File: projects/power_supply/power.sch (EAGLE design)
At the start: 82 parts, among them SW1 SRIDE_SWITCH, SW2 SRIDE_SWITCH, SW3 SRIDE_SWITCH, SW4 SRIDE_SWITCH, SW5 SRIDE_SWITCH, SW6 SRIDE_SWITCH, SW7 SRIDE_SWITCH, SW8 SRIDE_SWITCH

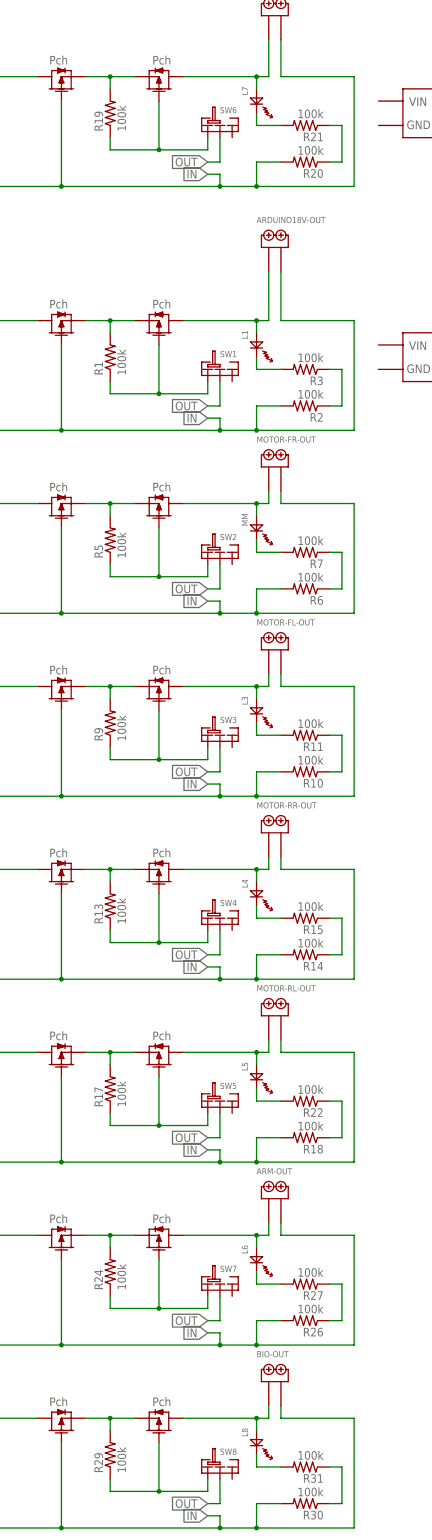
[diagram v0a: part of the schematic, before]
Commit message: power
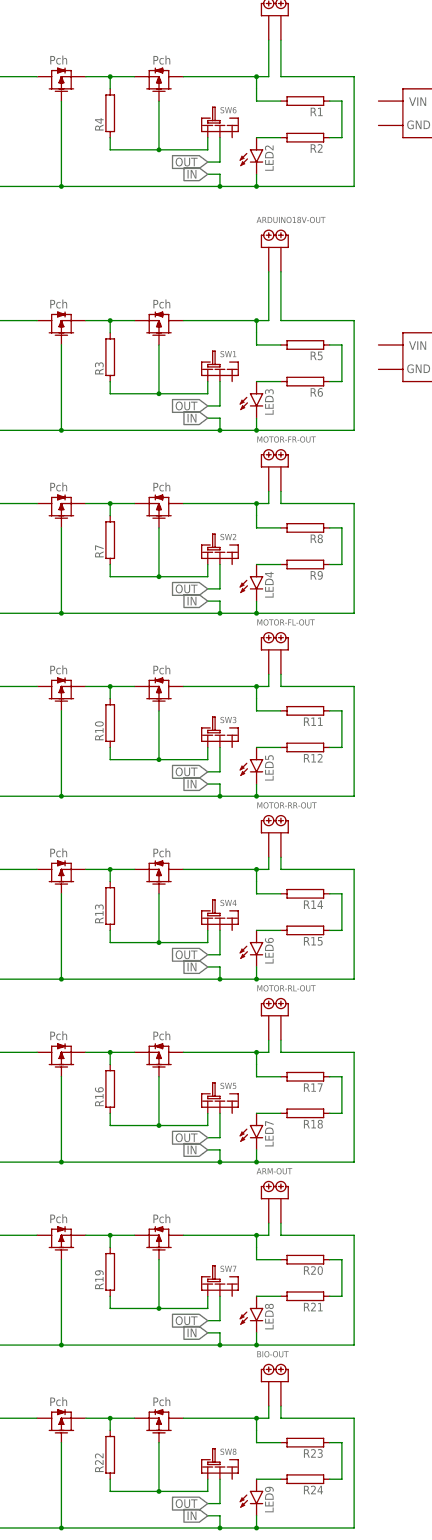
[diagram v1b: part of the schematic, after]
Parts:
- removed L1, L3, L4, L5, L6, L7, L8, MM: (no value), Chip LED:OSXX1608C1A
- removed R26, R27, R29, R30, R31: 100k, rcl:R-US_R0603
- added LED2, LED3, LED4, LED5, LED6, LED7, LED8, LED9: (no value), led:LED5MM
- added R12, R16, R23, R4, R8: (no value), resistor-power:RAC01
- R1, R10, R11, R13, R14, R15, R17, R18, R19, R2, R20, R21, R22, R24, R3, R5, R6, R7, R9: value 100k -> (none); device rcl:R-US_R0603 -> resistor-power:RAC01
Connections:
- removed net N$14: MM.CT, R7.2
- removed net N$23: L3.CT, R11.2
- removed net N$32: L4.CT, R15.2
- removed net N$41: L5.CT, R22.2
- removed net N$48: L7.CT, R21.2
- removed net N$5: L1.CT, R3.2
- removed net N$50: L8.CT, R31.2
- removed net N$56: L6.CT, R27.2
- removed net N$60 (its old number): R26.1, R27.1
- new net N$11: LED6.A, R15.2
- new net N$12: LED7.A, R18.2
- new net N$16: LED8.A, R21.2
- new net N$17: LED9.A, R24.2
- new net N$2: LED2.A, R2.2
- new net N$3: LED3.A, R6.2
- new net N$4: LED4.A, R9.2
- new net N$49: R1.1, R2.1
- new net N$7: LED5.A, R12.2
- net IN: now also LED2.C, LED3.C, LED4.C, LED5.C, LED6.C, LED7.C, LED8.C, LED9.C; no longer R10.2, R14.2, R18.2, R2.2, R20.2, R26.2, R30.2, R6.2
- net MA: now also R4.2; no longer R19.2
- net MAC: now also R1.2; no longer L7.AN
- net MCX: now also R16.2; no longer R17.2
- net MH: now also R10.2; no longer R9.2
- net MHGF: now also R20.2; no longer L6.AN
- net MHH: now also R14.2; no longer L4.AN
- net MHHHH: now also R23.2; no longer L8.AN
- net MJUY: now also R22.2; no longer R29.2
- net MKK: now also R3.2; no longer R1.2
- net MOO: now also R5.2; no longer L1.AN
- net MS: now also R7.2; no longer R5.2
- net MV: now also R11.2; no longer L3.AN
- net MVVV: now also R19.2; no longer R24.2
- net MZZ: now also R17.2; no longer L5.AN
- net N$1: now also R3.1; no longer R1.1
- net N$10: now also R7.1; no longer R5.1
- net N$13: now also R8.2; no longer MM.AN
- net N$15: now also R8.1, R9.1; no longer R6.1, R7.1
- net N$19: now also R10.1; no longer R9.1
- net N$24: now also R12.1; no longer R10.1
- net N$37: now also R16.1; no longer R17.1
- net N$42: now also R17.1; no longer R22.1
- net N$43: now also R4.1; no longer R19.1
- net N$52: now also R19.1; no longer R24.1
- net N$58: now also R23.1, R24.1; no longer R30.1, R31.1
- net N$6: now also R5.1, R6.1; no longer R2.1, R3.1
- net N$8: now also R22.1; no longer R29.1
